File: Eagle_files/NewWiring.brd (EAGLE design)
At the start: 103.8 x 85.1 mm, 60 parts, among them T1 PIN, T2 PIN

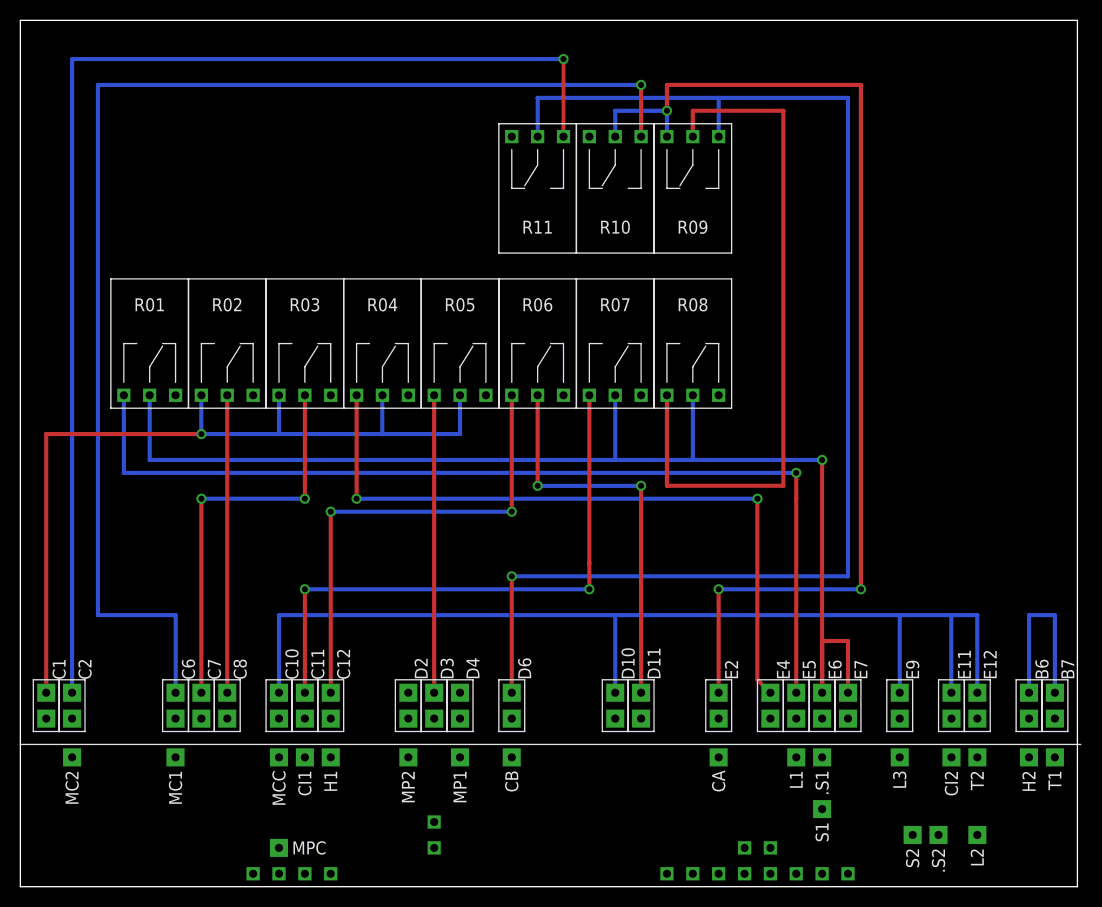
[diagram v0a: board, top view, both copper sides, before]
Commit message: Modified
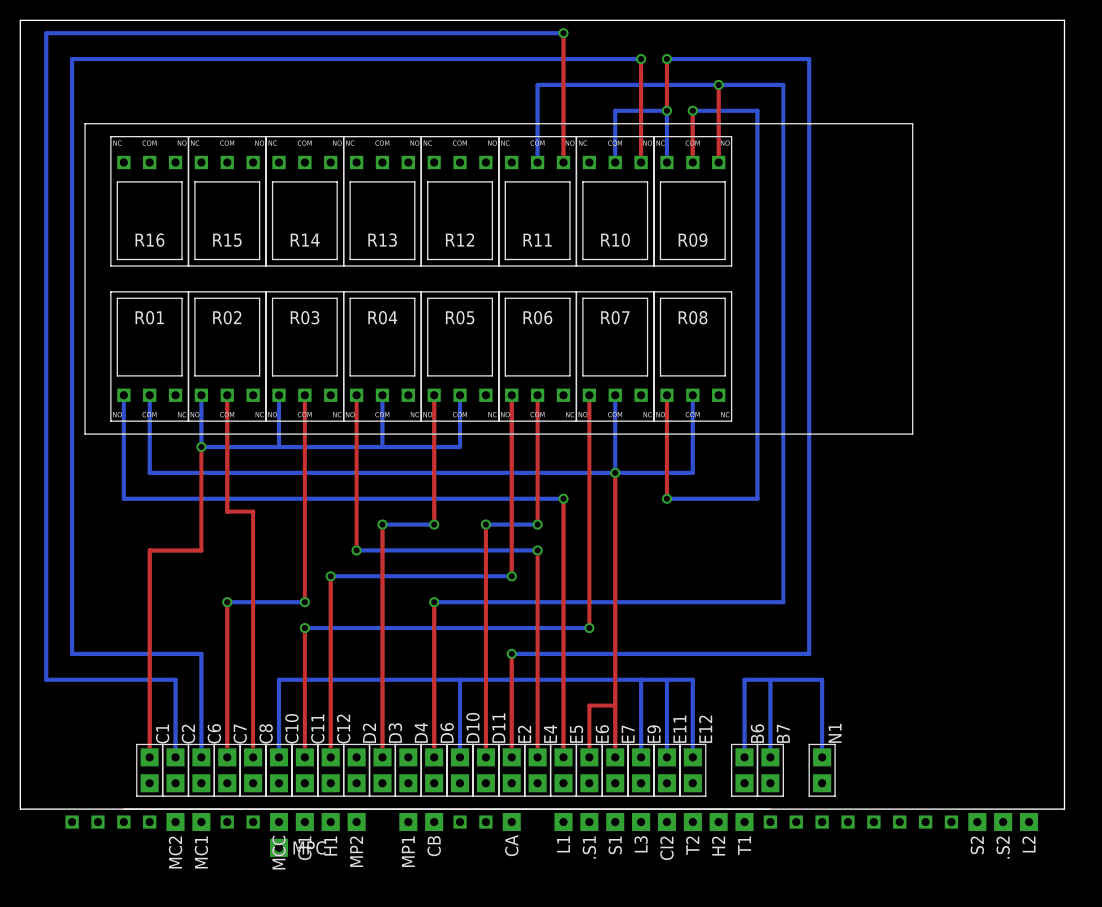
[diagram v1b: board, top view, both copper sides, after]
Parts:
- added N1: CABLE, Kostas:CABLE
- added R12, R13, R14, R15, R16: RELAY, Kostas:RELAY
- moved H2 31.1 mm to (68.6, 6.35)
- moved T1 31.1 mm to (71.1, 6.35)
- moved B6 28.7 mm to (71.1, 12.7)
- moved B7 28.7 mm to (73.7, 12.7)
- moved CI2 28.7 mm to (63.5, 6.35)
- moved E11 28.7 mm to (63.5, 12.7)
- moved E12 28.7 mm to (66.0, 12.7)
- moved T2 28.7 mm to (66.0, 6.35)
- moved COLD_WATER_VALVE 28.1 mm to (43.2, 6.35)
- moved E9 26.2 mm to (61.0, 12.7)
- moved L3 26.2 mm to (61.0, 6.35)
- moved E4 23.7 mm to (50.8, 12.7)
- moved E5 23.7 mm to (53.3, 12.7)
- moved E7 23.7 mm to (58.4, 12.7)
- moved L1 23.7 mm to (53.3, 6.35)
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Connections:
- new net N$5: B6.P$1, B7.P$1, N1.P$1
- net D10: no longer HOT_WATER_VALVE.P$1
- net N$13: now also HOT_WATER_VALVE.P$1, N1.P$2; no longer B6.P$1, B7.P$1
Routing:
- net N$5: track 0.00 -> 30.5 mm
- net N$9: track 118.1 -> 147.3 mm
- net LIVE: track 106.7 -> 78.7 mm
- net N$16: track 105.4 -> 132.1 mm
- net N$11: track 125.7 -> 147.3 mm
- net N$13: track 17.8 -> 0.00 mm
- net N$6: track 95.2 -> 78.7 mm
- net N$47: track 69.1 -> 53.3 mm
- net N$25: track 29.2 -> 40.6 mm, vias 0 -> 2
- net N$15: track 129.5 -> 139.7 mm, vias 1 -> 2
- net NEUTRAL: track 120.7 -> 111.8 mm
- net N$42: track 29.2 -> 38.1 mm
- net N$23: track 47.0 -> 53.3 mm
- net N$24: track 57.1 -> 63.5 mm
- net N$43: track 39.4 -> 43.2 mm
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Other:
- board size 103.8 x 85.1 mm -> 102.5 x 77.5 mm
